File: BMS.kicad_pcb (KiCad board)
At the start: 4 copper layers, 30 x 70 mm, 111 parts, among them J8 Conn_01x03_Pin, Q1 FZT853TA, Q2 PSMN020-100YS, Q3 PSMN3R7-100BSE, SW1 SW_Push, SW2 SW_Push, U1 RP2350A, U4 MP2790DFP-0000-T, X1 ABM8-272-T3

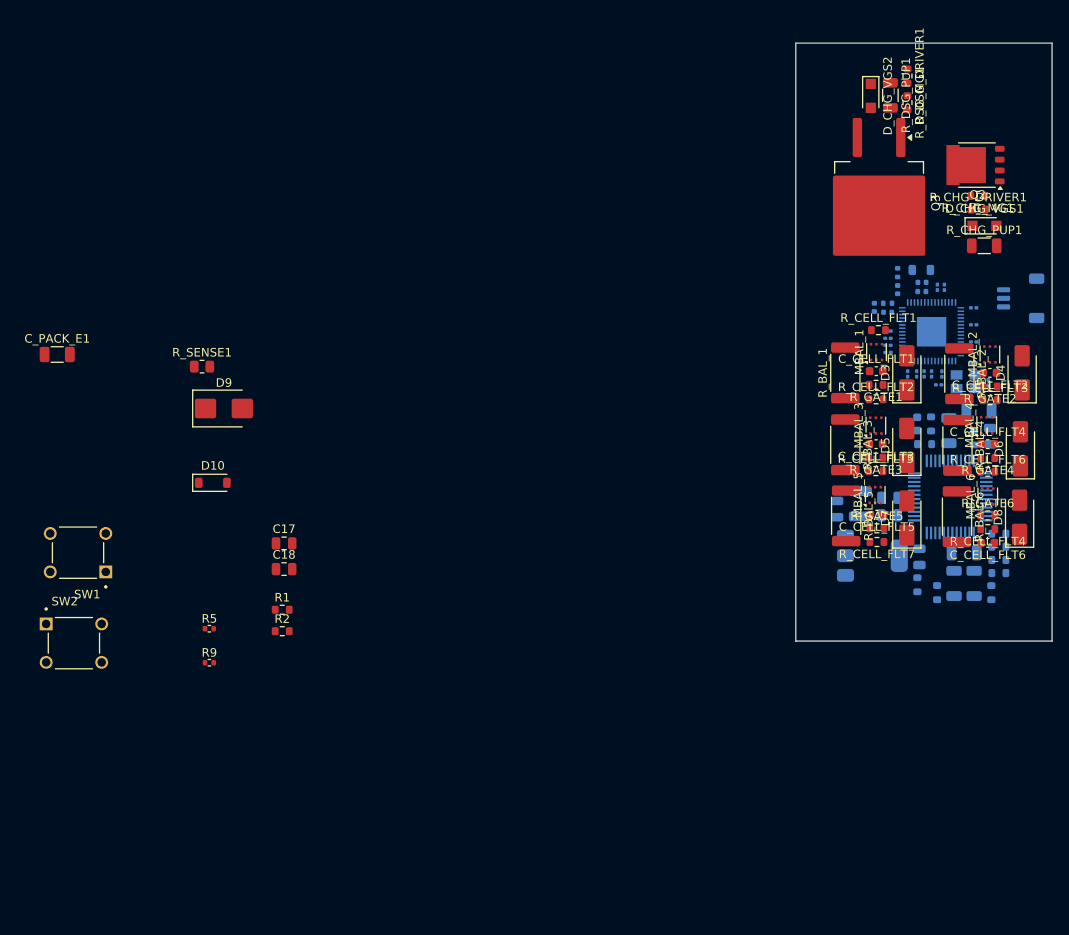
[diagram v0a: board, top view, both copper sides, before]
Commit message: Layed on board. Still need to route
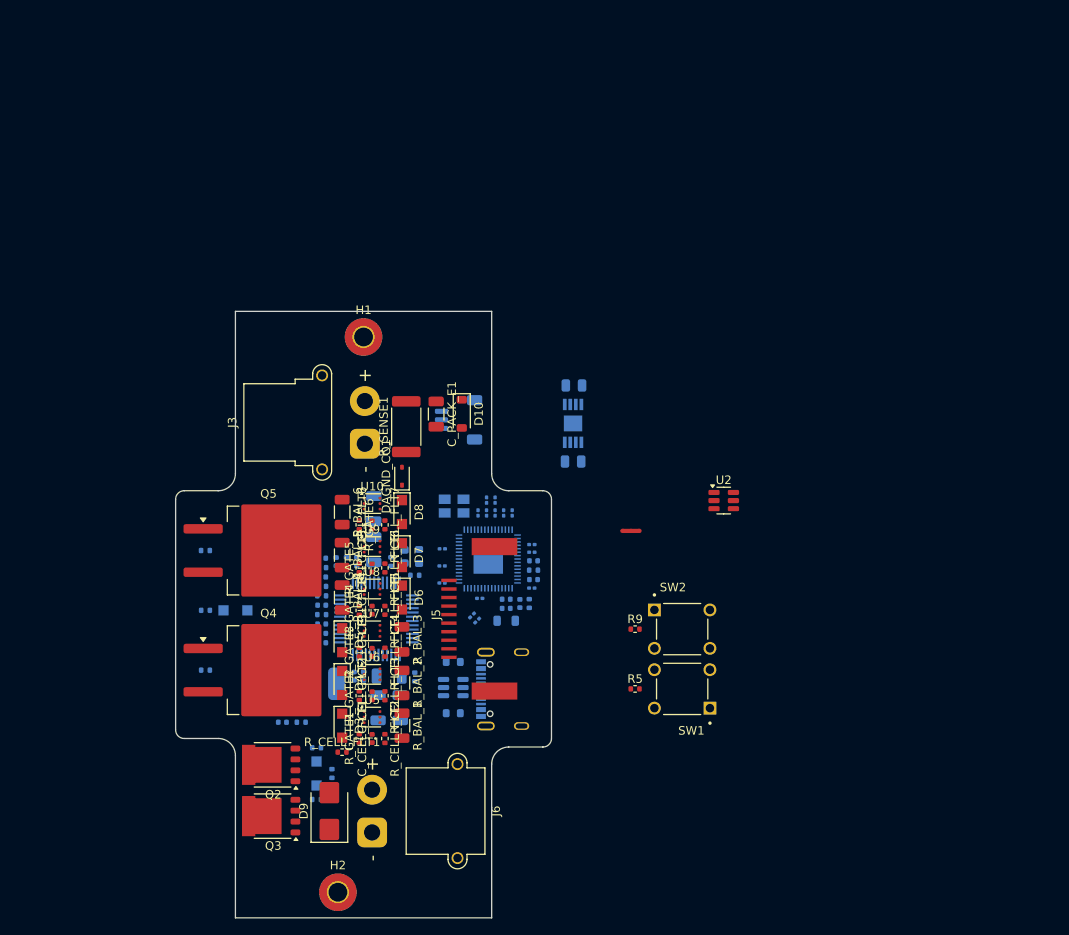
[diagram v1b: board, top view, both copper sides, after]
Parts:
- removed C17: 10uF, Capacitor_SMD:C_0805_2012Metric
- removed the C4 at (217.6, 70.7)
- removed MBAL_1, MBAL_2, MBAL_3, MBAL_4, MBAL_5, MBAL_6: MOSFET, _BMS:SC70-6
- added C19: 10n, Capacitor_SMD:C_0402_1005Metric, B.Cu at (145.0, 97.8)
- added C20: 10n, Capacitor_SMD:C_0402_1005Metric, B.Cu at (145.0, 94.5)
- added C21: 10n, Capacitor_SMD:C_0402_1005Metric, B.Cu at (145.0, 92.3)
- added C22: 10uF, Capacitor_SMD:C_0805_2012Metric, B.Cu at (174.5, 72.1)
- added C23: 10uF, Capacitor_SMD:C_0805_2012Metric, B.Cu at (174.4, 81.0)
- added DAGND_CO1: 4.7V 200MW, Diode_SMD:D_SOD-323, F.Cu at (154.4, 82.7)
- added H1: MountingHole, MountingHole:MountingHole_2.2mm_M2_Pad_TopBottom, F.Cu at (149.9, 66.4)
- added H2: MountingHole, MountingHole:MountingHole_2.2mm_M2_Pad_TopBottom, F.Cu at (146.9, 131.4)
- added J1: 12402012E212A, _BMS:AMPHENOL_12402012E212A, B.Cu at (168.4, 107.6)
- added J3: Conn_01x02_Socket, Connector_AMASS:AMASS_XT30PW-F_1x02_P2.50mm_Horizontal, F.Cu at (150.1, 78.9)
- added J5: Conn_01x10_Pin, _BMS:TB4-Hirose, F.Cu at (158.9, 98.9)
- added J6: Conn_01x02_Pin, Connector_AMASS:AMASS_XT30PW-M_1x02_P2.50mm_Horizontal, F.Cu at (150.9, 124.4)
- added NT1: NetTie_2, NetTie:NetTie-3_SMD_Pad0.5mm, F.Cu at (181.2, 89.1)
- added Q4: PSMN3R7-100BSE, _BMS:TO-263-2, F.Cu at (138.8, 105.4)
- added Q5: PSMN3R7-100BSE, _BMS:TO-263-2, F.Cu at (138.8, 91.4)
- added R_CHG_MG2: 100 Ω, Resistor_SMD:R_0402_1005Metric, B.Cu at (144.4, 120.5)
- added R_DSG_MG2: 100 Ω, Resistor_SMD:R_0402_1005Metric, B.Cu at (131.4, 105.4)
- added U1: USBLC6-2SC6, Package_TO_SOT_SMD:SOT-23-6, B.Cu at (160.4, 107.4)
- added U10: SQ1464EEH-T1_GE3, _BMS:SC70-6, F.Cu at (150.9, 85.9)
- added U12: TPS7B8133QDGNRQ1, _BMS:VSSOP8_DGN_TEX, B.Cu at (174.4, 76.5)
- added U2: USBLC6-2SC6, Package_TO_SOT_SMD:SOT-23-6, F.Cu at (192.1, 85.5)
- added U5: SQ1464EEH-T1_GE3, _BMS:SC70-6, F.Cu at (150.9, 110.9)
- added U6: SQ1464EEH-T1_GE3, _BMS:SC70-6, F.Cu at (150.9, 105.9)
- added U7: SQ1464EEH-T1_GE3, _BMS:SC70-6, F.Cu at (150.9, 100.8)
- added U8: SQ1464EEH-T1_GE3, _BMS:SC70-6, F.Cu at (150.9, 95.9)
- added U9: SQ1464EEH-T1_GE3, _BMS:SC70-6, F.Cu at (150.9, 90.9)
- C18: value 10uF -> 10n; footprint Capacitor_SMD:C_0805_2012Metric -> Capacitor_SMD:C_0402_1005Metric; moved to B.Cu
- C_3V1, C_REG1, C_VDD1, C_VREF1: footprint Capacitor_SMD:C_0805_2012Metric -> Capacitor_SMD:C_0402_1005Metric
- C_CELL_FLT1, C_CELL_FLT2, C_CELL_FLT3, C_CELL_FLT4, C_CELL_FLT5, C_CELL_FLT6, C_PACK_FLT1: value 10 nF -> 10n; footprint Capacitor_SMD:C_0603_1608Metric -> Capacitor_SMD:C_0402_1005Metric
- C_REGIN1: footprint Capacitor_SMD:C_1210_3225Metric -> Capacitor_SMD:C_0603_1608Metric
- C_TOP_FLT1: footprint Capacitor_SMD:C_0805_2012Metric -> Capacitor_SMD:C_0603_1608Metric
- D3, D4, D5, D6, D7, D8: value D_Zener -> PTVS5V0S1UR,115; footprint Diode_SMD:D_SMA -> Diode_SMD:Nexperia_CFP3_SOD-123W
- D_CHG_VGS1, D_CHG_VGS2, R1, R2: moved to B.Cu
- Q2: footprint Package_TO_SOT_SMD:LFPAK56 -> _BMS:LFPAK56_1
- Q3: value PSMN3R7-100BSE -> PSMN020-100YS; footprint Package_TO_SOT_SMD:TO-263-2 -> _BMS:LFPAK56_1
- R13, R14, R15, R16, R_CELL_FLT1, R_CELL_FLT2, R_CELL_FLT3, R_CELL_FLT4, R_CELL_FLT5, R_CELL_FLT6, R_CELL_FLT7, R_GATE1, R_GATE2, R_GATE3, R_GATE4, R_GATE5, R_GATE6, R_PACK_FLT1, R_REG1, R_SRN_FLT1, R_SRP_FLT1, R_TOP_FLT1: footprint Resistor_SMD:R_0603_1608Metric -> Resistor_SMD:R_0402_1005Metric
- R_BAL_1, R_BAL_2, R_BAL_3, R_BAL_4, R_BAL_5, R_BAL_6: footprint Resistor_SMD:R_2512_6332Metric -> Resistor_SMD:R_1206_3216Metric
- R_CHG_DRIVER1, R_CHG_MG1, R_DSG_DRIVER1, R_DSG_MG1: footprint Resistor_SMD:R_0603_1608Metric -> Resistor_SMD:R_0402_1005Metric; moved to B.Cu
- R_CHG_PUP1, R_DSG_PUP1: footprint Resistor_SMD:R_1206_3216Metric -> Resistor_SMD:R_0402_1005Metric; moved to B.Cu
- R_SENSE1: footprint Resistor_SMD:R_0805_2012Metric -> Resistor_SMD:R_2512_6332Metric
- moved Q2 108.3 mm to (139.2, 116.5)
- moved D_CHG_VGS1 101.1 mm to (144.4, 117.5), turned to -90 degrees
- moved Q3 101.0 mm to (139.2, 122.5), turned to 180 degrees
- moved R_CHG_MG1 100.8 mm to (144.4, 114.5), turned to 0 degrees
- moved R_DSG_PUP1 100.3 mm to (131.4, 98.4), turned to 0 degrees
- moved R_CHG_PUP1 98.2 mm to (146.2, 117.5), turned to -90 degrees
- moved R_DSG_MG1 97.5 mm to (131.4, 91.4), turned to 0 degrees
- moved D_CHG_VGS2 95.7 mm to (134.9, 98.4), turned to 180 degrees
- moved D4 87.5 mm to (147.4, 106.9), turned to -90 degrees
- moved R_DSG_DRIVER1 86.0 mm to (149.1, 92.7), turned to 90 degrees
- moved R_GATE2 82.2 mm to (149.4, 108.4), turned to 90 degrees
- moved C_CELL_FLT2 81.6 mm to (150.9, 108.4), turned to 90 degrees
- moved R_CHG_DRIVER1 80.2 mm to (153.1, 92.7), turned to 90 degrees
- moved R_CELL_FLT1 79.9 mm to (147.4, 115.0)
- moved R13 79.8 mm to (145.0, 98.9), turned to 180 degrees
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- renumbered C11 to C10, C12 to C11, C13 to C12, C14 to C13, C15 to C14, C16 to C15, C5 to C4, C6 to C5, C7 to C6, C8 to C7, C9 to C8, C10 to C9, J8 to J4, U4 to U11, U1 to U3
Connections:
- C18 pad 1: +3V3 -> GNDREF
- C18 pad 2: GND -> /main/BMS/NTC4
- C_3V1 pad 1: /main/BMS/AGND -> Net-(U11-3V3)
- C_3V1 pad 2: Net-(U4-3V3) -> GNDREF
- C_MID1 pad 2: /main/BMS/AGND -> GNDREF
- C_PACK_E1 pad 1: /main/BMS/BATT+ -> /main/BMS/PACK+
- C_PACK_E1 pad 2: /main/BMS/PGNDE -> GND
- C_PACK_FLT1 pad 1: /main/BMS/AGND -> Net-(U11-PACKP)
- C_PACK_FLT1 pad 2: Net-(U4-PACKP) -> GNDREF
- C_REG1 pad 2: /main/BMS/AGND -> GNDREF
- C_REGIN1 pad 1: /main/BMS/AGND -> GNDREF
- C_SRN_GND1 pad 1: /main/BMS/AGND -> GNDREF
- C_SRP_GND1 pad 2: /main/BMS/AGND -> GNDREF
- C_TOP_FLT1 pad 2: /main/BMS/AGND -> GNDREF
- C_VDD1 pad 2: /main/BMS/AGND -> GNDREF
- C_VREF1 pad 1: /main/BMS/AGND -> GNDREF
- D10 pad 1: /main/BMS/BATT+ -> /main/BMS/PACK+
- D10 pad 2: /main/BMS/PGNDE -> GND
- D_CHG_VGS2 pad 2: /main/BMS/BATT+ -> /main/BMS/PACK+
- Q3 pad 3: /main/BMS/BATT+ -> /main/BMS/TOP
- R11 pad 2: /main/external_io/D+ -> /main/external_io/D-
- R13 pad 2: /main/BMS/AGND -> GNDREF
- R14 pad 2: /main/BMS/AGND -> GNDREF
- R15 pad 2: /main/BMS/AGND -> GNDREF
- R16 pad 2: /main/BMS/AGND -> GNDREF
- R_CELL_FLT4 pad 1: GND -> /main/BMS/C3
- R_CELL_FLT4 pad 2: /main/BMS/CELL_0 -> /main/BMS/CELL_3
- R_CELL_FLT5 pad 1: /main/BMS/C3 -> /main/BMS/C2
- R_CELL_FLT5 pad 2: /main/BMS/CELL_3 -> /main/BMS/CELL_2
- R_CELL_FLT6 pad 1: /main/BMS/C2 -> /main/BMS/C1
- R_CELL_FLT6 pad 2: /main/BMS/CELL_2 -> /main/BMS/CELL_1
- R_CELL_FLT7 pad 1: /main/BMS/C1 -> GND
- R_CELL_FLT7 pad 2: /main/BMS/CELL_1 -> /main/BMS/CELL_0
- R_DSG_MG1 pad 2: Net-(Q3-G) -> Net-(Q5-G)
- R_DSG_PUP1 pad 2: /main/BMS/BATT+ -> /main/BMS/PACK+
- R_PACK_FLT1 pad 1: Net-(U4-PACKP) -> Net-(U11-PACKP)
- R_SENSE1 pad 2: /main/BMS/PGNDE -> /main/BMS/PACK-
- R_SRN_FLT1 pad 2: /main/BMS/PGNDE -> /main/BMS/PACK-
- U11 pad 21: /main/BMS/AGND -> GNDREF
- U11 pad 23: /main/BMS/AGND -> GNDREF
- U11 pad 26: Net-(U4-3V3) -> Net-(U11-3V3)
- U11 pad 38: Net-(U4-PACKP) -> Net-(U11-PACKP)
- U3 pad 20: +3V3 -> unconnected-(U3-IOVDD-Pad20)
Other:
- board size 30 x 70 mm -> 44 x 71 mm
